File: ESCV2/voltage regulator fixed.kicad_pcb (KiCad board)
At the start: 4 copper layers, 45.2 x 85.2 mm, 39 parts

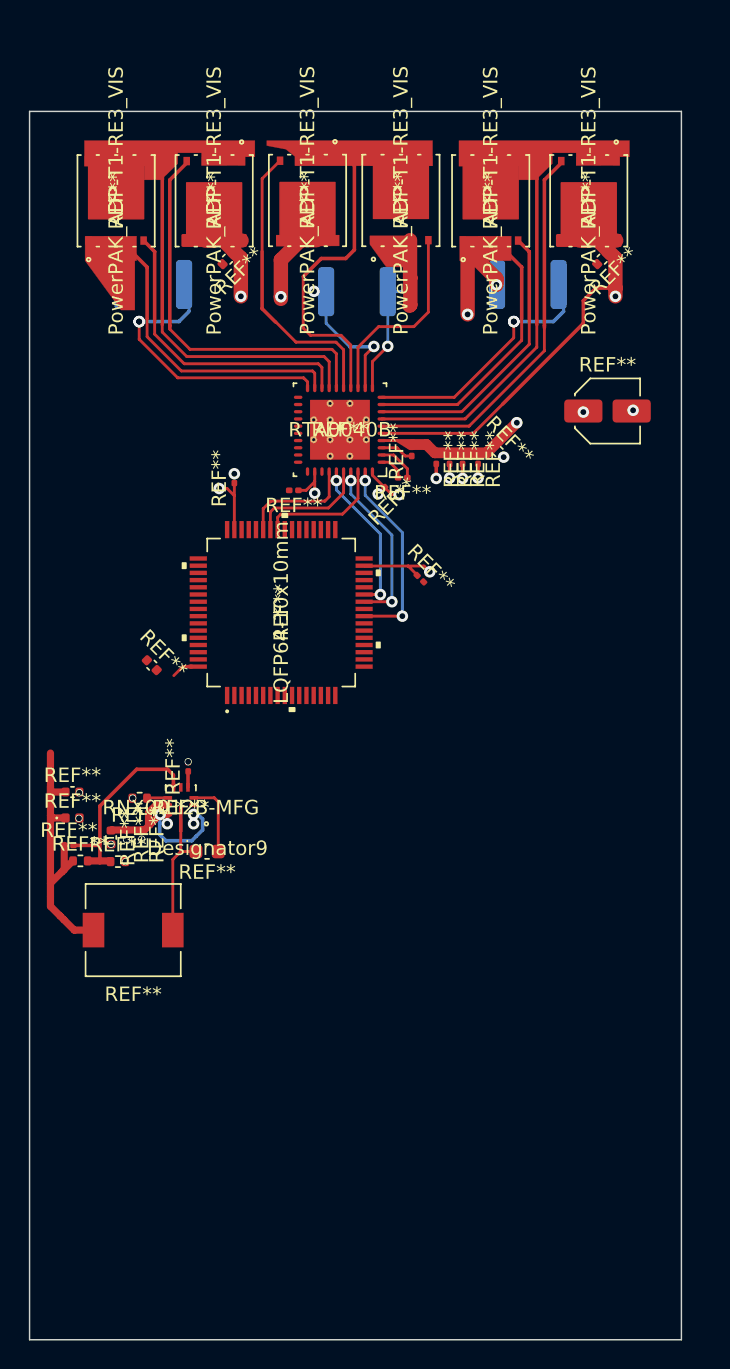
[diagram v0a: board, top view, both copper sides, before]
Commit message: l
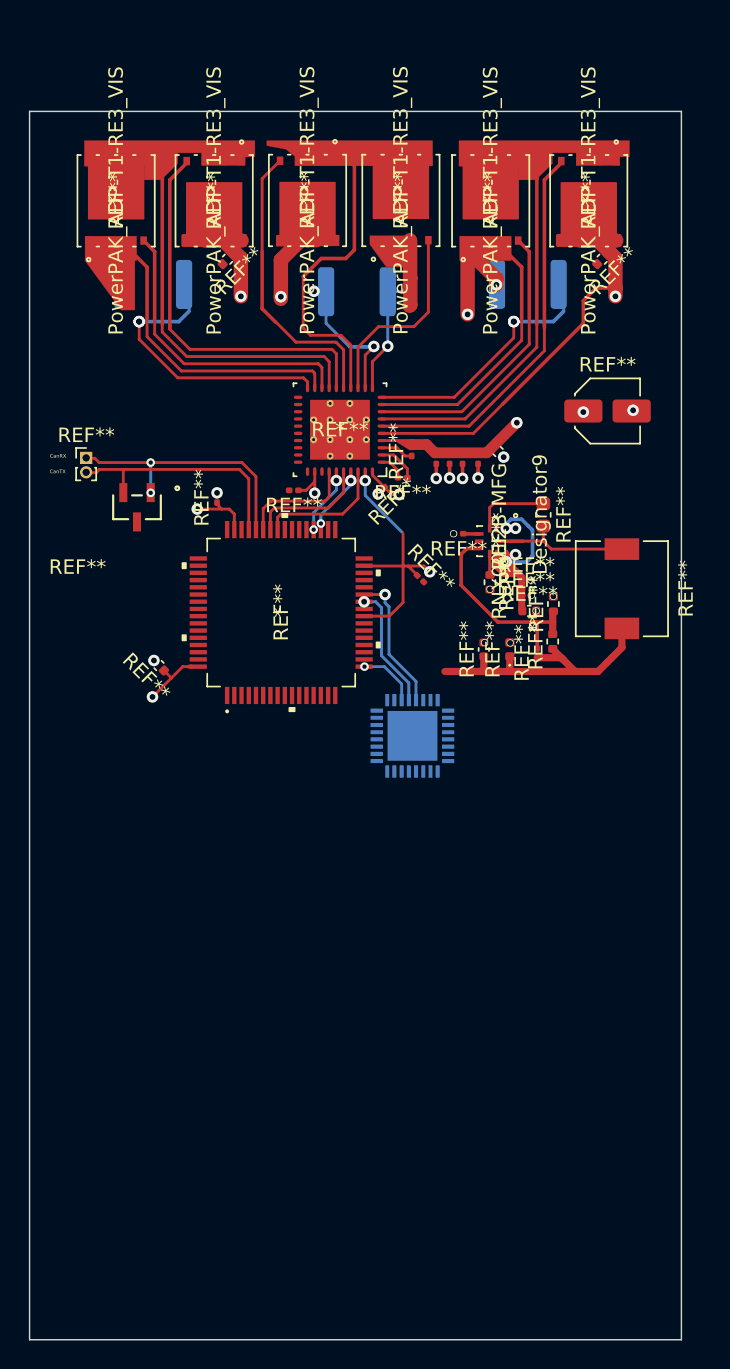
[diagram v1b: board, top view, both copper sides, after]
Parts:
- added REF**: PinHeader_1x02_P1.00mm_Vertical, Connector_PinHeader_1.00mm:PinHeader_1x02_P1.00mm_Vertical, F.Cu at (146.7, 88.8)
- added REF**: SOT-23_DBZ_TEX, PESD2CAN24DBZRQ1:PESD2CAN24DBZRQ1, F.Cu at (150.2, 92.2)
- added REF**: RHB32_3P45X3P45_TEX, TEXASusb:TUSB1210BRHBRQ1, B.Cu at (169.3, 108.1)
- moved REF** 41.3 mm to (183.8, 97.9), turned to -90 degrees
- moved REF** 36.1 mm to (179.1, 101.6), turned to 90 degrees
- moved REF** 35.1 mm to (178.0, 102.4), turned to 90 degrees
- moved REF** 35.1 mm to (179.1, 99.0), turned to 90 degrees
- moved REF** 33.0 mm to (178.4, 92.8), turned to -90 degrees
- moved REF** 33.0 mm to (177.4, 99.4), turned to 0 degrees
- moved REF** 32.5 mm to (176.1, 102.1), turned to 90 degrees
- moved REF** 32.3 mm to (177.2, 98.4), turned to 0 degrees
- moved REF** 32.0 mm to (177.2, 97.3), turned to 0 degrees
- moved REF** 30.2 mm to (174.3, 102.1), turned to 90 degrees
- moved REF** 28.8 mm to (175.4, 94.6), turned to -90 degrees
- moved REF** 28.5 mm to (174.7, 97.5), turned to -90 degrees
- moved REF** 24.8 mm to (172.5, 94.1), turned to 180 degrees
- moved REF** 1.81 mm to (155.8, 91.6)
- moved REF** 0.50 mm to (151.8, 103.2), turned to 135 degrees
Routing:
- net (no net): track 517.2 -> 562.8 mm, vias 44 -> 50
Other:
- board text added: "CanRX"
- board text added: "CanTX"
